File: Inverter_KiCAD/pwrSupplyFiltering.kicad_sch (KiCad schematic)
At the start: 8 parts

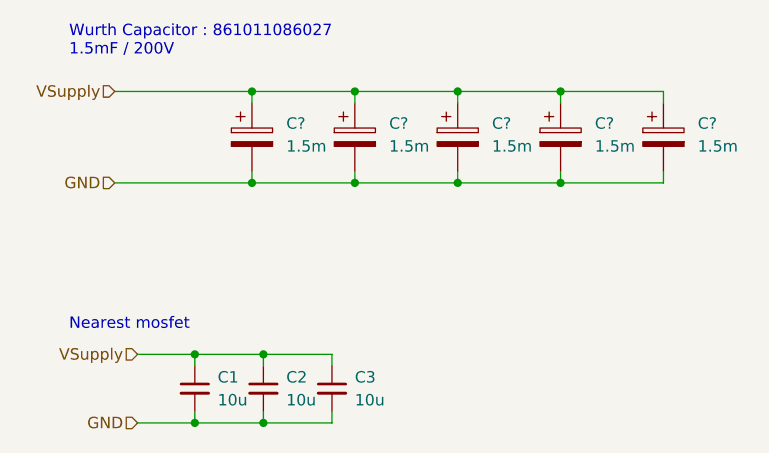
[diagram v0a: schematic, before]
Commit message: v0 PCB
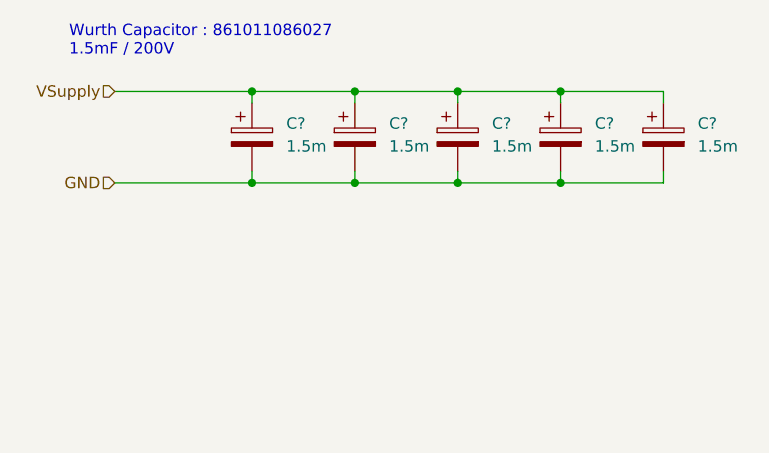
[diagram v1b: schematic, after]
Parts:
- removed C1, C2, C3: 10u, Capacitor_SMD:C_0805_2012Metric, symbol Device:C_Small
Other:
- note removed: "Nearest mosfet"
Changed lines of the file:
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@@
   (junction (at 147.32 68.58) (diameter 0) (color 0 0 0 0)
-  )
-  (junction (at 118.11 95.25) (diameter 0) (color 0 0 0 0)
-  )
-  (junction (at 125.73 95.25) (diameter 0) (color 0 0 0 0)
   )
   (junction (at 124.46 58.42) (diameter 0) (color 0 0 0 0)
@@
   (junction (at 135.89 58.42) (diameter 0) (color 0 0 0 0)
   )
-  (junction (at 118.11 87.63) (diameter 0) (color 0 0 0 0)
-  )
   (junction (at 147.32 58.42) (diameter 0) (color 0 0 0 0)
-  )
-  (junction (at 125.73 87.63) (diameter 0) (color 0 0 0 0)
   )
   (junction (at 124.46 68.58) (diameter 0) (color 0 0 0 0)
@@
     (stroke (width 0) (type default))
   )
-  (wire (pts (xy 118.11 87.63) (xy 125.73 87.63))
-    (stroke (width 0) (type default))
-  )
   (wire (pts (xy 109.22 68.58) (xy 124.46 68.58))
-    (stroke (width 0) (type default))
-  )
-  (wire (pts (xy 133.35 95.25) (xy 133.35 93.98))
     (stroke (width 0) (type default))
   )
@@
   )
   (wire (pts (xy 124.46 67.31) (xy 124.46 68.58))
-    (stroke (width 0) (type default))
-  )
-  (wire (pts (xy 118.11 93.98) (xy 118.11 95.25))
-    (stroke (width 0) (type default))
-  )
-  (wire (pts (xy 118.11 87.63) (xy 118.11 88.9))
     (stroke (width 0) (type default))
   )
@@
     (stroke (width 0) (type default))
   )
-  (wire (pts (xy 133.35 88.9) (xy 133.35 87.63))
-    (stroke (width 0) (type default))
-  )
   (wire (pts (xy 170.18 59.69) (xy 170.18 58.42))
-    (stroke (width 0) (type default))
-  )
-  (wire (pts (xy 111.76 87.63) (xy 118.11 87.63))
-    (stroke (width 0) (type default))
-  )
-  (wire (pts (xy 133.35 87.63) (xy 125.73 87.63))
     (stroke (width 0) (type default))
   )
@@
     (stroke (width 0) (type default))
   )
-  (wire (pts (xy 125.73 93.98) (xy 125.73 95.25))
-    (stroke (width 0) (type default))
-  )
   (wire (pts (xy 170.18 67.31) (xy 170.18 68.58))
     (stroke (width 0) (type default))
@@
     (stroke (width 0) (type default))
   )
-  (wire (pts (xy 125.73 88.9) (xy 125.73 87.63))
-    (stroke (width 0) (type default))
-  )
-  (wire (pts (xy 118.11 95.25) (xy 125.73 95.25))
-    (stroke (width 0) (type default))
-  )
-  (wire (pts (xy 125.73 95.25) (xy 133.35 95.25))
-    (stroke (width 0) (type default))
-  )
-  (wire (pts (xy 111.76 95.25) (xy 118.11 95.25))
-    (stroke (width 0) (type default))
-  )
   (text "Wurth Capacitor : 861011086027\n1.5mF / 200V" (at 104.14 54.61 0)
-    (effects (font (size 1.27 1.27)) (justify left bottom))
-  )
-  (text "Nearest mosfet" (at 104.14 85.09 0)
     (effects (font (size 1.27 1.27)) (justify left bottom))
   )
@@
     (effects (font (size 1.27 1.27)) (justify right))
   )
-  (hierarchical_label "VSupply" (shape input) (at 111.76 87.63 180) (fields_autoplaced)
-    (effects (font (size 1.27 1.27)) (justify right))
-  )
-  (hierarchical_label "GND" (shape input) (at 111.76 95.25 180) (fields_autoplaced)
-    (effects (font (size 1.27 1.27)) (justify right))
-  )
   (hierarchical_label "GND" (shape input) (at 109.22 68.58 180) (fields_autoplaced)
     (effects (font (size 1.27 1.27)) (justify right))
-  )
-  (symbol (lib_id "Device:C_Small") (at 125.73 91.44 0) (unit 1)
-    (in_bom yes) (on_board yes) (dnp no) (fields_autoplaced)
-    (property "Reference" "C2" (at 128.27 90.1763 0)
-      (effects (font (size 1.27 1.27)) (justify left))
-    )
-    (property "Value" "10u" (at 128.27 92.7163 0)
-      (effects (font (size 1.27 1.27)) (justify left))
-    )
-    (property "Footprint" "Capacitor_SMD:C_0805_2012Metric" (at 125.73 91.44 0)
-      (effects (font (size 1.27 1.27)) hide)
-    )
-    (property "Datasheet" "~" (at 125.73 91.44 0)
-      (effects (font (size 1.27 1.27)) hide)
-    )
-    (pin "1")
-    (pin "2")
-    (instances
-      (project "Inverter_KiCAD"
-        (path "/5e6c1e3f-0815-454a-8acb-8e3e2d064875/3abd505c-2b96-4cc2-9359-42e0642ca937"
-          (reference "C2") (unit 1)
-        )
-      )
-    )
-  )
-  (symbol (lib_id "Device:C_Small") (at 133.35 91.44 0) (unit 1)
-    (in_bom yes) (on_board yes) (dnp no) (fields_autoplaced)
-    (property "Reference" "C3" (at 135.89 90.1763 0)
-      (effects (font (size 1.27 1.27)) (justify left))
-    )
-    (property "Value" "10u" (at 135.89 92.7163 0)
-      (effects (font (size 1.27 1.27)) (justify left))
-    )
-    (property "Footprint" "Capacitor_SMD:C_0805_2012Metric" (at 133.35 91.44 0)
-      (effects (font (size 1.27 1.27)) hide)
-    )
-    (property "Datasheet" "~" (at 133.35 91.44 0)
-      (effects (font (size 1.27 1.27)) hide)
-    )
-    (pin "1")
-    (pin "2")
-    (instances
-      (project "Inverter_KiCAD"
-        (path "/5e6c1e3f-0815-454a-8acb-8e3e2d064875/3abd505c-2b96-4cc2-9359-42e0642ca937"
-          (reference "C3") (unit 1)
-        )
-      )
-    )
   )
   (symbol (lib_id "Device:C_Polarized") (at 135.89 63.5 0) (unit 1)
@@
         )
       )
-    )
-  )
-  (symbol (lib_id "Device:C_Small") (at 118.11 91.44 0) (unit 1)
-    (in_bom yes) (on_board yes) (dnp no) (fields_autoplaced)
-    (property "Reference" "C1" (at 120.65 90.1763 0)
-      (effects (font (size 1.27 1.27)) (justify left))
-    )
-    (property "Value" "10u" (at 120.65 92.7163 0)
-      (effects (font (size 1.27 1.27)) (justify left))
-    )
-    (property "Footprint" "Capacitor_SMD:C_0805_2012Metric" (at 118.11 91.44 0)
-      (effects (font (size 1.27 1.27)) hide)
-    )
-    (property "Datasheet" "~" (at 118.11 91.44 0)
-      (effects (font (size 1.27 1.27)) hide)
-    )
-    (pin "1")
-    (pin "2")
-    (instances
-      (project "Inverter_KiCAD"
-        (path "/5e6c1e3f-0815-454a-8acb-8e3e2d064875/3abd505c-2b96-4cc2-9359-42e0642ca937"
-          (reference "C1") (unit 1)
-        )
-      )

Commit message: change pbs
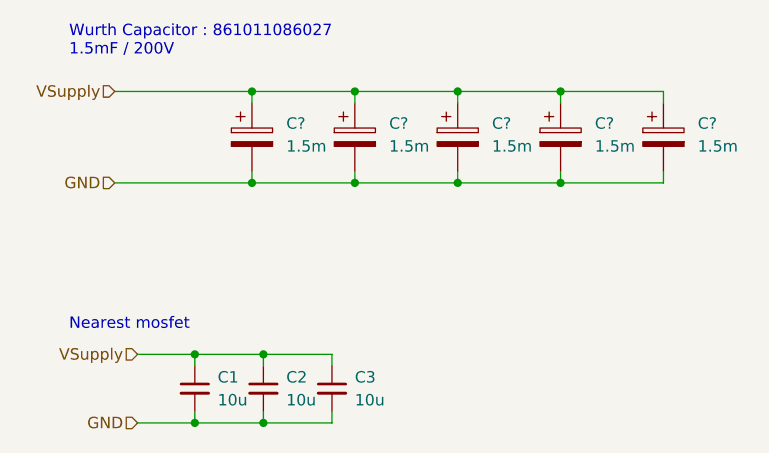
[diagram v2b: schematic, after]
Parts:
- added C1, C2, C3: 10u, Capacitor_SMD:C_0805_2012Metric, symbol Device:C_Small
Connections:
- net GND: now also C1.2, C2.2, C3.2
- net VSupply: now also C1.1, C2.1, C3.1
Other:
- note added: "Nearest mosfet"
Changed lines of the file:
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@@
   (junction (at 147.32 68.58) (diameter 0) (color 0 0 0 0)
   )
+  (junction (at 118.11 95.25) (diameter 0) (color 0 0 0 0)
+  )
+  (junction (at 125.73 95.25) (diameter 0) (color 0 0 0 0)
+  )
   (junction (at 124.46 58.42) (diameter 0) (color 0 0 0 0)
   )
@@
   (junction (at 135.89 58.42) (diameter 0) (color 0 0 0 0)
   )
+  (junction (at 118.11 87.63) (diameter 0) (color 0 0 0 0)
+  )
   (junction (at 147.32 58.42) (diameter 0) (color 0 0 0 0)
   )
+  (junction (at 125.73 87.63) (diameter 0) (color 0 0 0 0)
+  )
   (junction (at 124.46 68.58) (diameter 0) (color 0 0 0 0)
   )
@@
     (stroke (width 0) (type default))
   )
+  (wire (pts (xy 118.11 87.63) (xy 125.73 87.63))
+    (stroke (width 0) (type default))
+  )
   (wire (pts (xy 109.22 68.58) (xy 124.46 68.58))
     (stroke (width 0) (type default))
   )
+  (wire (pts (xy 133.35 95.25) (xy 133.35 93.98))
+    (stroke (width 0) (type default))
+  )
   (wire (pts (xy 158.75 58.42) (xy 158.75 59.69))
     (stroke (width 0) (type default))
@@
     (stroke (width 0) (type default))
   )
+  (wire (pts (xy 118.11 93.98) (xy 118.11 95.25))
+    (stroke (width 0) (type default))
+  )
+  (wire (pts (xy 118.11 87.63) (xy 118.11 88.9))
+    (stroke (width 0) (type default))
+  )
   (wire (pts (xy 147.32 68.58) (xy 158.75 68.58))
     (stroke (width 0) (type default))
@@
     (stroke (width 0) (type default))
   )
+  (wire (pts (xy 133.35 88.9) (xy 133.35 87.63))
+    (stroke (width 0) (type default))
+  )
   (wire (pts (xy 170.18 59.69) (xy 170.18 58.42))
     (stroke (width 0) (type default))
   )
+  (wire (pts (xy 111.76 87.63) (xy 118.11 87.63))
+    (stroke (width 0) (type default))
+  )
+  (wire (pts (xy 133.35 87.63) (xy 125.73 87.63))
+    (stroke (width 0) (type default))
+  )
   (wire (pts (xy 124.46 68.58) (xy 135.89 68.58))
     (stroke (width 0) (type default))
@@
     (stroke (width 0) (type default))
   )
+  (wire (pts (xy 125.73 93.98) (xy 125.73 95.25))
+    (stroke (width 0) (type default))
+  )
   (wire (pts (xy 170.18 67.31) (xy 170.18 68.58))
     (stroke (width 0) (type default))
@@
   )
   (wire (pts (xy 158.75 68.58) (xy 170.18 68.58))
+    (stroke (width 0) (type default))
+  )
+  (wire (pts (xy 125.73 88.9) (xy 125.73 87.63))
+    (stroke (width 0) (type default))
+  )
+  (wire (pts (xy 118.11 95.25) (xy 125.73 95.25))
+    (stroke (width 0) (type default))
+  )
+  (wire (pts (xy 125.73 95.25) (xy 133.35 95.25))
+    (stroke (width 0) (type default))
+  )
+  (wire (pts (xy 111.76 95.25) (xy 118.11 95.25))
     (stroke (width 0) (type default))
   )
@@
     (effects (font (size 1.27 1.27)) (justify left bottom))
   )
+  (text "Nearest mosfet" (at 104.14 85.09 0)
+    (effects (font (size 1.27 1.27)) (justify left bottom))
+  )
   (hierarchical_label "VSupply" (shape input) (at 109.22 58.42 180) (fields_autoplaced)
     (effects (font (size 1.27 1.27)) (justify right))
   )
+  (hierarchical_label "VSupply" (shape input) (at 111.76 87.63 180) (fields_autoplaced)
+    (effects (font (size 1.27 1.27)) (justify right))
+  )
+  (hierarchical_label "GND" (shape input) (at 111.76 95.25 180) (fields_autoplaced)
+    (effects (font (size 1.27 1.27)) (justify right))
+  )
   (hierarchical_label "GND" (shape input) (at 109.22 68.58 180) (fields_autoplaced)
     (effects (font (size 1.27 1.27)) (justify right))
+  )
+  (symbol (lib_id "Device:C_Small") (at 125.73 91.44 0) (unit 1)
+    (in_bom yes) (on_board yes) (dnp no) (fields_autoplaced)
+    (property "Reference" "C2" (at 128.27 90.1763 0)
+      (effects (font (size 1.27 1.27)) (justify left))
+    )
+    (property "Value" "10u" (at 128.27 92.7163 0)
+      (effects (font (size 1.27 1.27)) (justify left))
+    )
+    (property "Footprint" "Capacitor_SMD:C_0805_2012Metric" (at 125.73 91.44 0)
+      (effects (font (size 1.27 1.27)) hide)
+    )
+    (property "Datasheet" "~" (at 125.73 91.44 0)
+      (effects (font (size 1.27 1.27)) hide)
+    )
+    (pin "1")
+    (pin "2")
+    (instances
+      (project "Inverter_KiCAD"
+        (path "/5e6c1e3f-0815-454a-8acb-8e3e2d064875/3abd505c-2b96-4cc2-9359-42e0642ca937"
+          (reference "C2") (unit 1)
+        )
+      )
+    )
+  )
+  (symbol (lib_id "Device:C_Small") (at 133.35 91.44 0) (unit 1)
+    (in_bom yes) (on_board yes) (dnp no) (fields_autoplaced)
+    (property "Reference" "C3" (at 135.89 90.1763 0)
+      (effects (font (size 1.27 1.27)) (justify left))
+    )
+    (property "Value" "10u" (at 135.89 92.7163 0)
+      (effects (font (size 1.27 1.27)) (justify left))
+    )
+    (property "Footprint" "Capacitor_SMD:C_0805_2012Metric" (at 133.35 91.44 0)
+      (effects (font (size 1.27 1.27)) hide)
+    )
+    (property "Datasheet" "~" (at 133.35 91.44 0)
+      (effects (font (size 1.27 1.27)) hide)
+    )
+    (pin "1")
+    (pin "2")
+    (instances
+      (project "Inverter_KiCAD"
+        (path "/5e6c1e3f-0815-454a-8acb-8e3e2d064875/3abd505c-2b96-4cc2-9359-42e0642ca937"
+          (reference "C3") (unit 1)
+        )
+      )
+    )
   )
   (symbol (lib_id "Device:C_Polarized") (at 135.89 63.5 0) (unit 1)
@@
         )
       )
+    )
+  )
+  (symbol (lib_id "Device:C_Small") (at 118.11 91.44 0) (unit 1)
+    (in_bom yes) (on_board yes) (dnp no) (fields_autoplaced)
+    (property "Reference" "C1" (at 120.65 90.1763 0)
+      (effects (font (size 1.27 1.27)) (justify left))
+    )
+    (property "Value" "10u" (at 120.65 92.7163 0)
+      (effects (font (size 1.27 1.27)) (justify left))
+    )
+    (property "Footprint" "Capacitor_SMD:C_0805_2012Metric" (at 118.11 91.44 0)
+      (effects (font (size 1.27 1.27)) hide)
+    )
+    (property "Datasheet" "~" (at 118.11 91.44 0)
+      (effects (font (size 1.27 1.27)) hide)
+    )
+    (pin "1")
+    (pin "2")
+    (instances
+      (project "Inverter_KiCAD"
+        (path "/5e6c1e3f-0815-454a-8acb-8e3e2d064875/3abd505c-2b96-4cc2-9359-42e0642ca937"
+          (reference "C1") (unit 1)
+        )
+      )
